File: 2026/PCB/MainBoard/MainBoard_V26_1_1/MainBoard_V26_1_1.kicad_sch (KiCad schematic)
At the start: 82 parts, among them J1 Raspberry_Pi_2_3, J11 //ADC2, J12 //ADC2, J13 //Drib, J14 UART, J15 TFT3, J16 CAN_CON, J2 fan, J4 metor, J6 Debug, J7 //ADC0, J8 MOLEX MINISPOX, Q1 Q_NMOS_GSD, Q2 Q_NMOS_GSD, SW1 SW_MEC_5E, SW2 Ras_1, SW3 Ras_2, SW4 SW_Wuerth_450301014042, SW5 SW_MEC_5E, SW6 SW_MEC_5E, U1 STM32F446RETx, U10 MPU9250, U2 LMR51460FSQDRRRQ1, U3 MOUDLE-SEEEDUINO-XIAO, U6 BNO055, U8 MAX3051, Y1 CSTNE16M0V530000R0

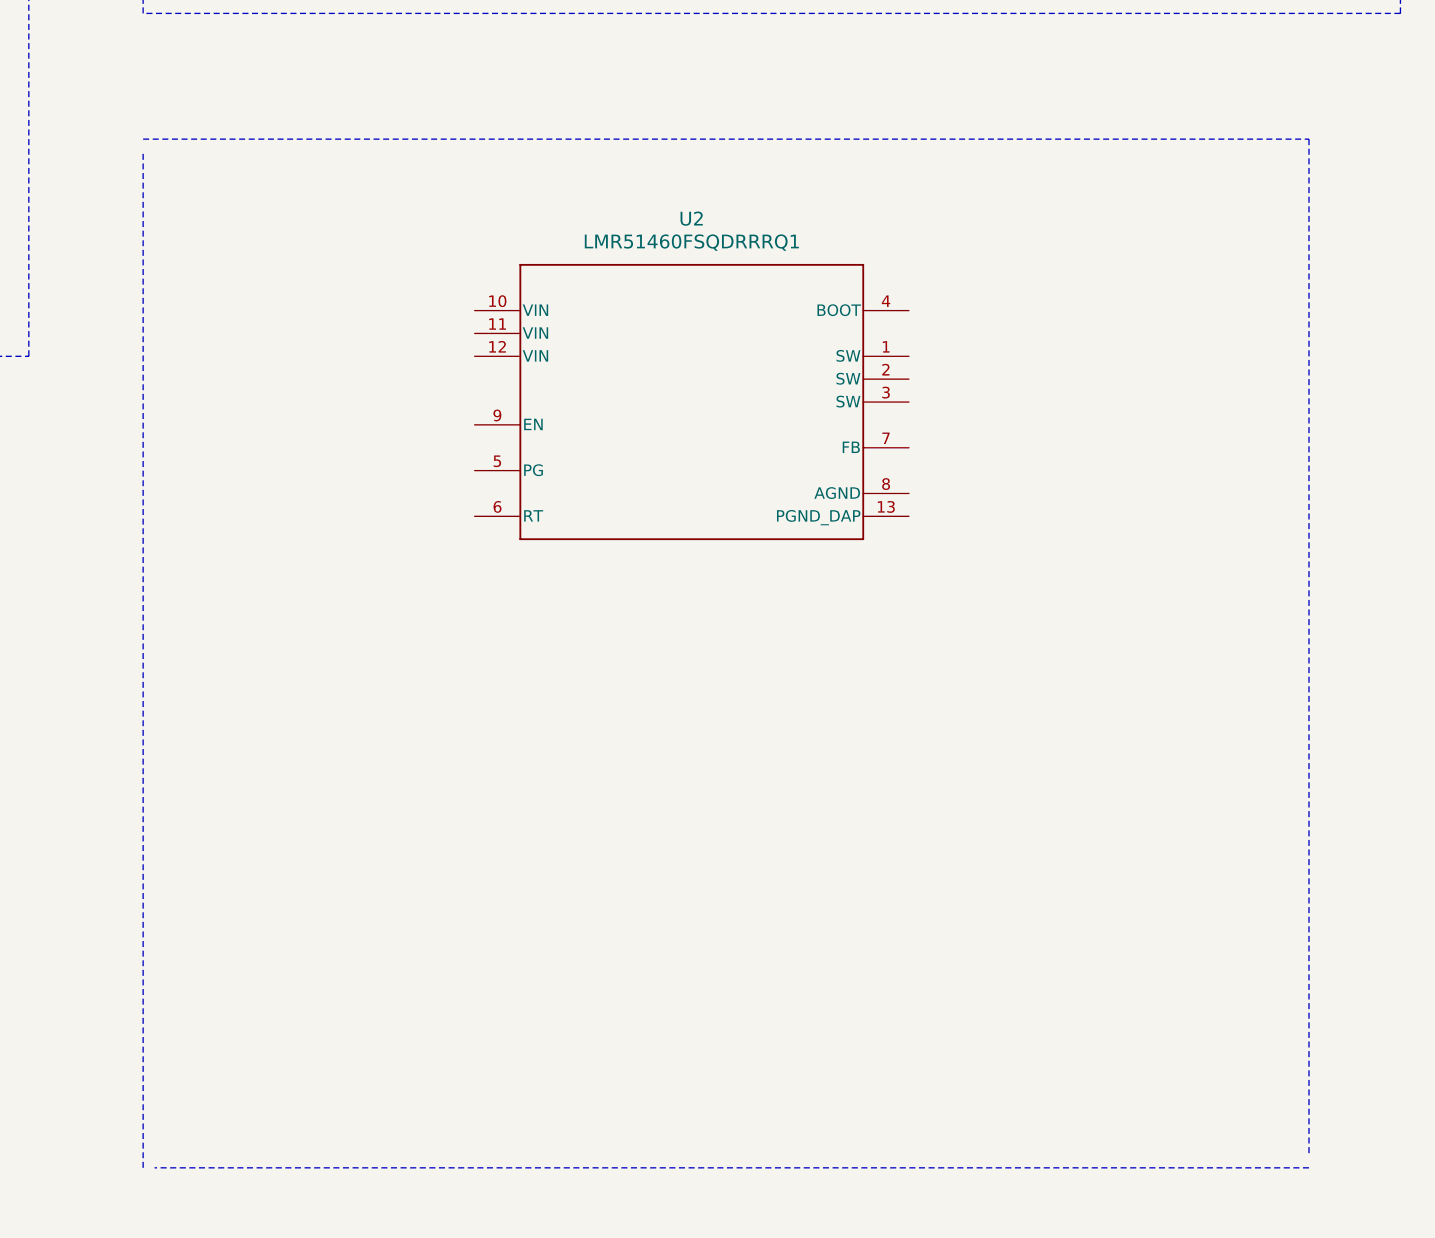
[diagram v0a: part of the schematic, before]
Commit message: 電源周りほぼ完成
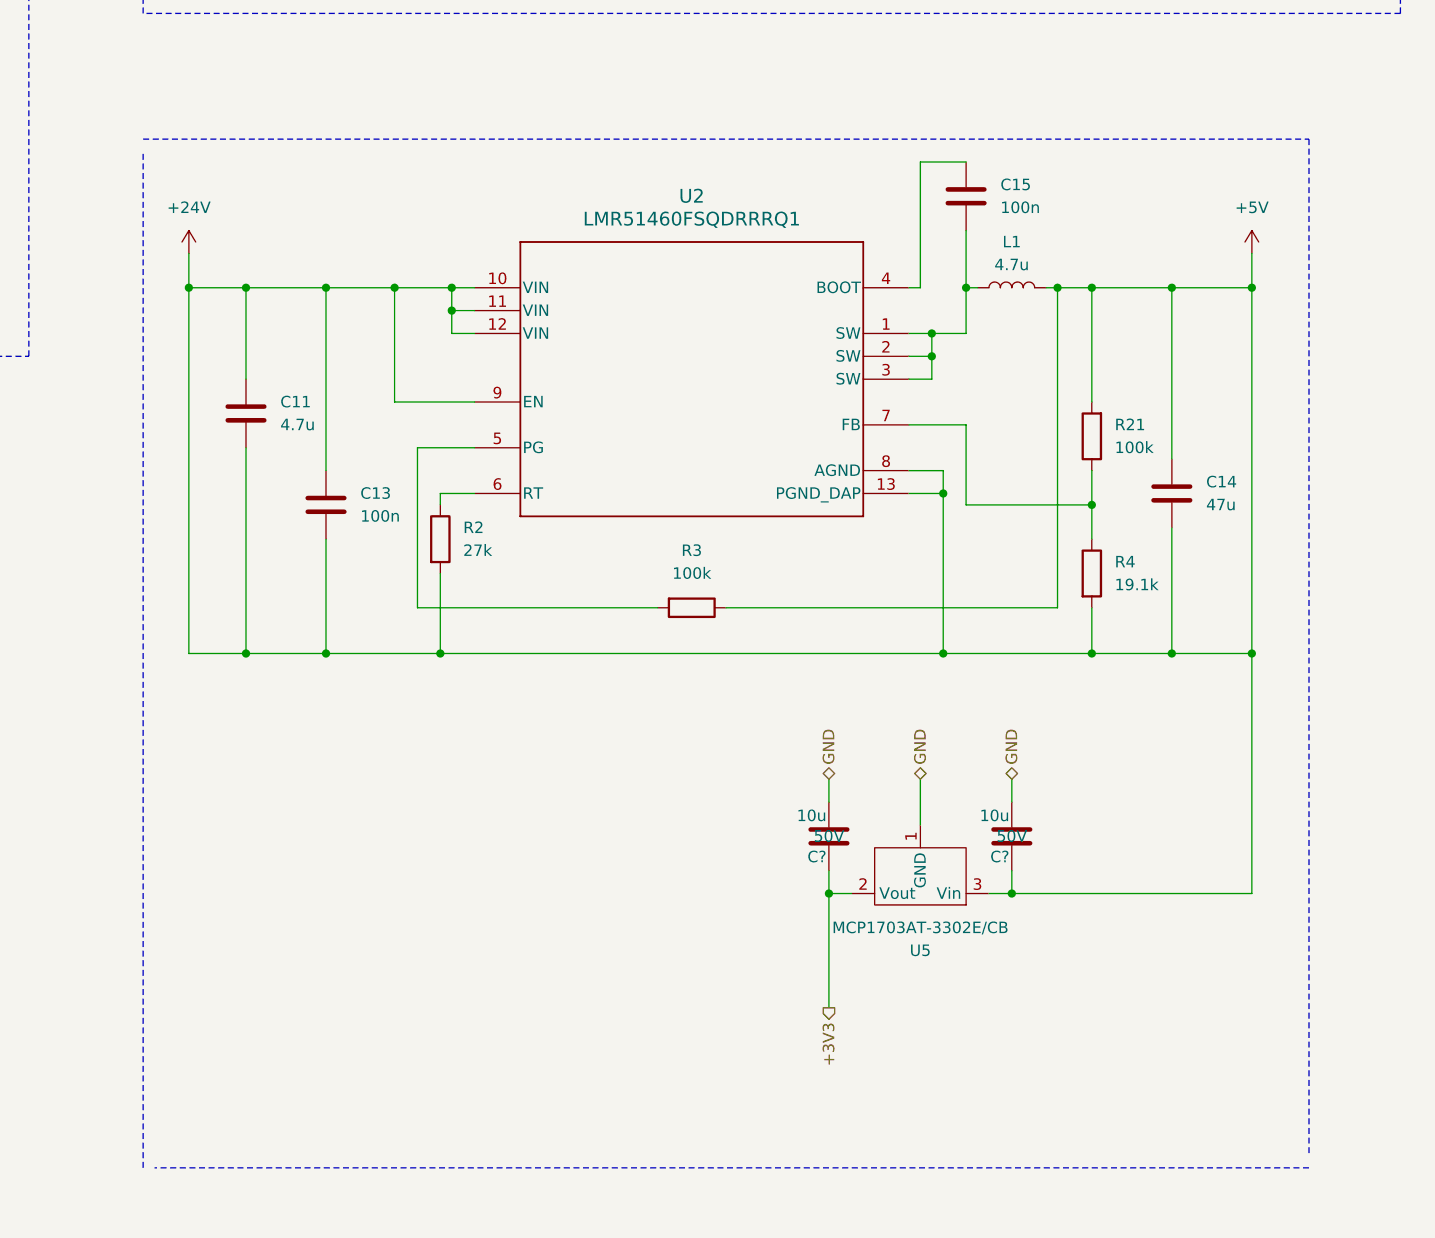
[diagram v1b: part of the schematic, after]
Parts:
- added C11: 4.7u, symbol Device:C
- added C13, C15: 100n, symbol Device:C
- added C14: 47u, symbol Device:C
- added C? (x2): 10u, Capacitor_SMD:C_0805_2012Metric_Pad1.18x1.45mm_HandSolder, symbol Device:C
- added L1: 4.7u, symbol Device:L
- added R2: 27k, symbol Device:R
- added R21, R3: 100k, symbol Device:R
- added R4: 19.1k, symbol Device:R
- added U5: MCP1703AT-3302E/CB, Package_TO_SOT_SMD:TSOT-23, symbol WheelVoltageBooster_LIB_SYM:MCP1703AT-3302E/CB
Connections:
- net +5V is gone; now on net +24V: C10.1, C12.1, C24.1, C9.1, D3.2 (A), J1.2 (5V), J1.4 (5V), J2.1 (Pin_1), U3.14 (5V)
- net GND: now also C?.2, C?.2, U5.1 (GND)
- net at U2.1 (SW): now also U2.2 (SW), U2.3 (SW), C15.2, L1.1
- net +24V: now reaches U2.10 (VIN)
- net +24V: now also U2.11 (VIN), U2.12 (VIN), U2.13 (PGND_DAP), U2.8 (AGND), U2.9 (EN), C11.1, C11.2, C13.1, C13.2, C14.1, C14.2, C?.1, L1.2, R2.2, R21.2, R3.1, R4.2, U5.3 (Vin)
- net at U2.4 (BOOT): now also C15.1
- net at U2.5 (PG): now also R3.2
- net at U2.6 (RT): now also R2.1
- net at U2.7 (FB): now also R21.1, R4.1
- new net +3V3: C?.1, U5.2 (Vout)
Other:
- moved on the sheet: U2
